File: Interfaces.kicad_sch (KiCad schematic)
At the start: 13 parts, among them J10 UART1_HDR, J11 UART2_HDR, J13 I2C1_Headers, J4 I/O_HDR, U8 TCA9517D

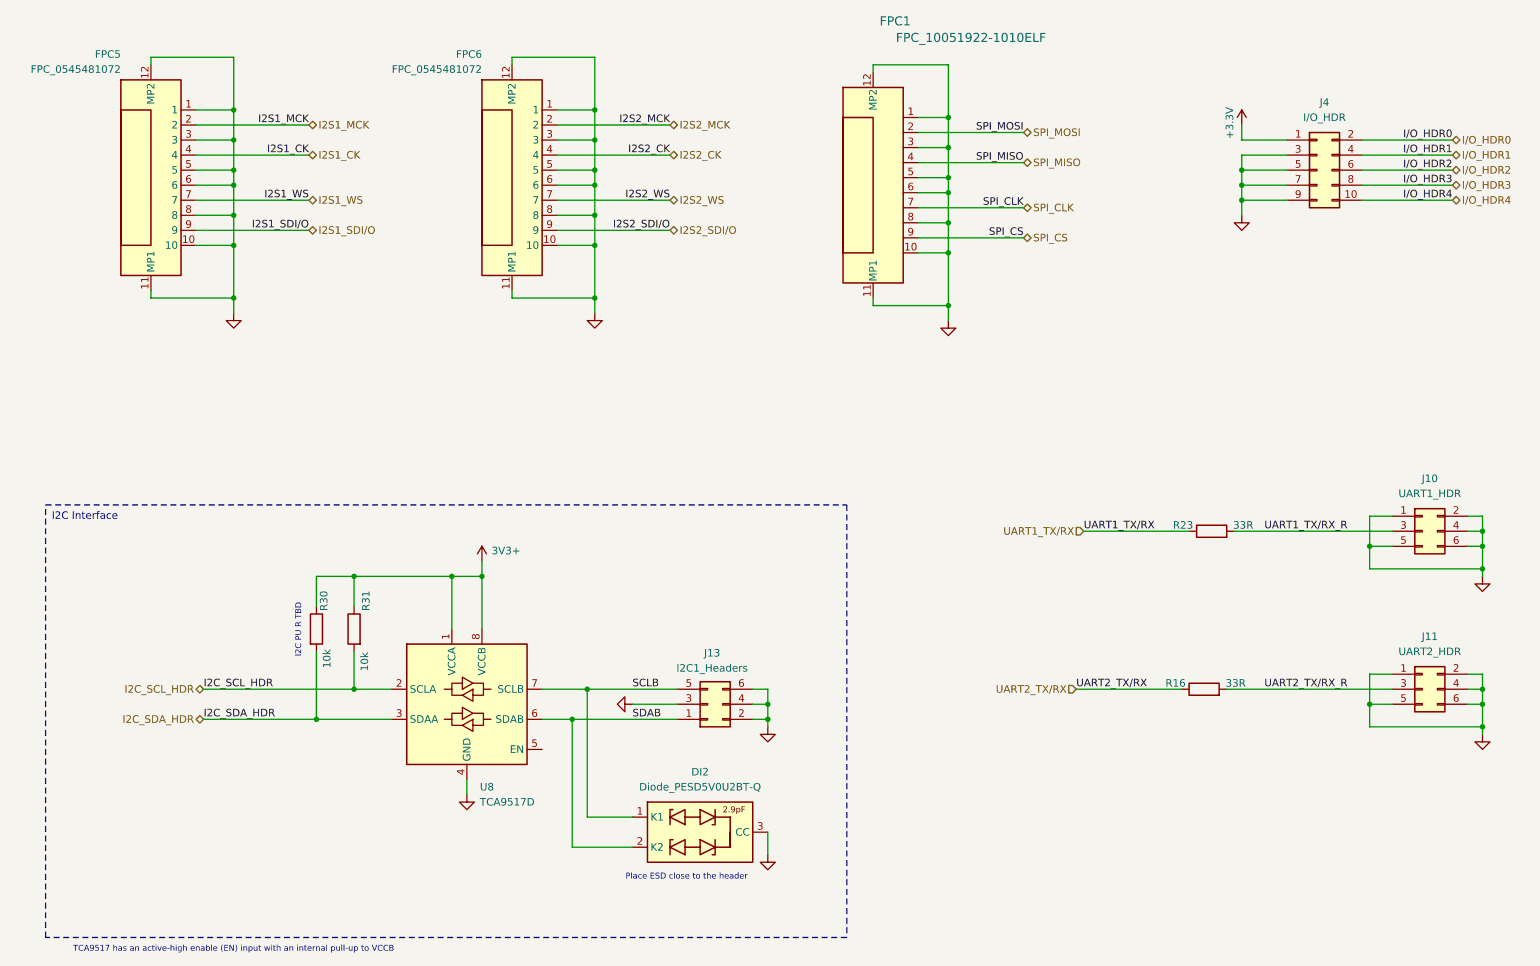
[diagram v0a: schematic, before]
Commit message: Interface Update
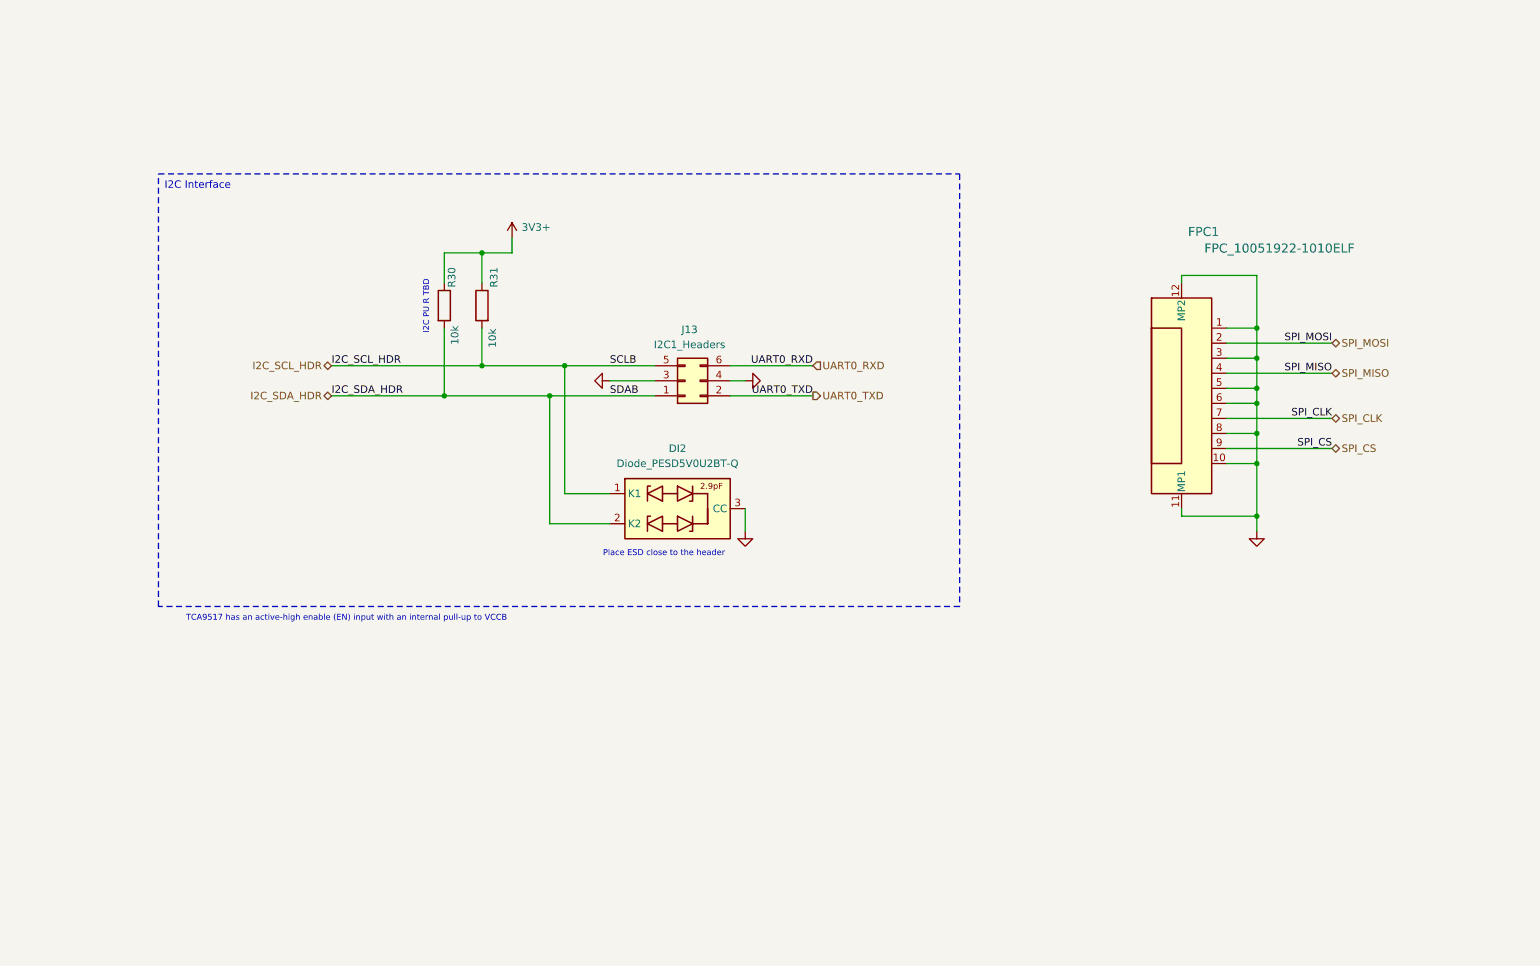
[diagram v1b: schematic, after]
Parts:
- removed FPC5, FPC6: FPC_0545481072, Personal_Project:FPC_10051922_1010, symbol Personal_Projects:FPC_0545481072
- removed J10: UART1_HDR, Personal_Project:PinHeader_2x03_P2.54mm_Horizontal_Court, symbol Connector_Generic:Conn_02x03_Odd_Even
- removed J11: UART2_HDR, Personal_Project:PinHeader_2x03_P2.54mm_Horizontal_Court, symbol Connector_Generic:Conn_02x03_Odd_Even
- removed J4: I/O_HDR, Connector_PinHeader_2.54mm:PinHeader_2x05_P2.54mm_Horizontal, symbol Connector_Generic:Conn_02x05_Odd_Even
- removed R16, R23: 33R, Resistor_SMD:R_0805_2012Metric, symbol Device:R
- removed U8: TCA9517D, Package_SO:SOIC-8_3.9x4.9mm_P1.27mm, symbol Logic_LevelTranslator:TCA9517D
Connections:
- net SCLB is gone; now on net I2C_SCL_HDR: DI2.1 (K1), J13.5 (Pin_5)
- net SDAB is gone; now on net I2C_SDA_HDR: DI2.2 (K2), J13.1 (Pin_1)
- net GND: no longer J13.2 (Pin_2), J13.6 (Pin_6)
- new net UART0_RXD: J13.6 (Pin_6)
- new net UART0_TXD: J13.2 (Pin_2)
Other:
- company: (none) -> Peter Hancak
- title: (none) -> ESP32P4C5_BOARD
- moved on the sheet: DI2, FPC1, J13, R30, R31
